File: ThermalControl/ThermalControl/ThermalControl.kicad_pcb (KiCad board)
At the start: 2 copper layers, 75 x 49 mm, 24 parts, among them J1 12V, J2 GND, J3 DC IN, J4 5V, U1 NODE_MCU, U2 RELAY MOD

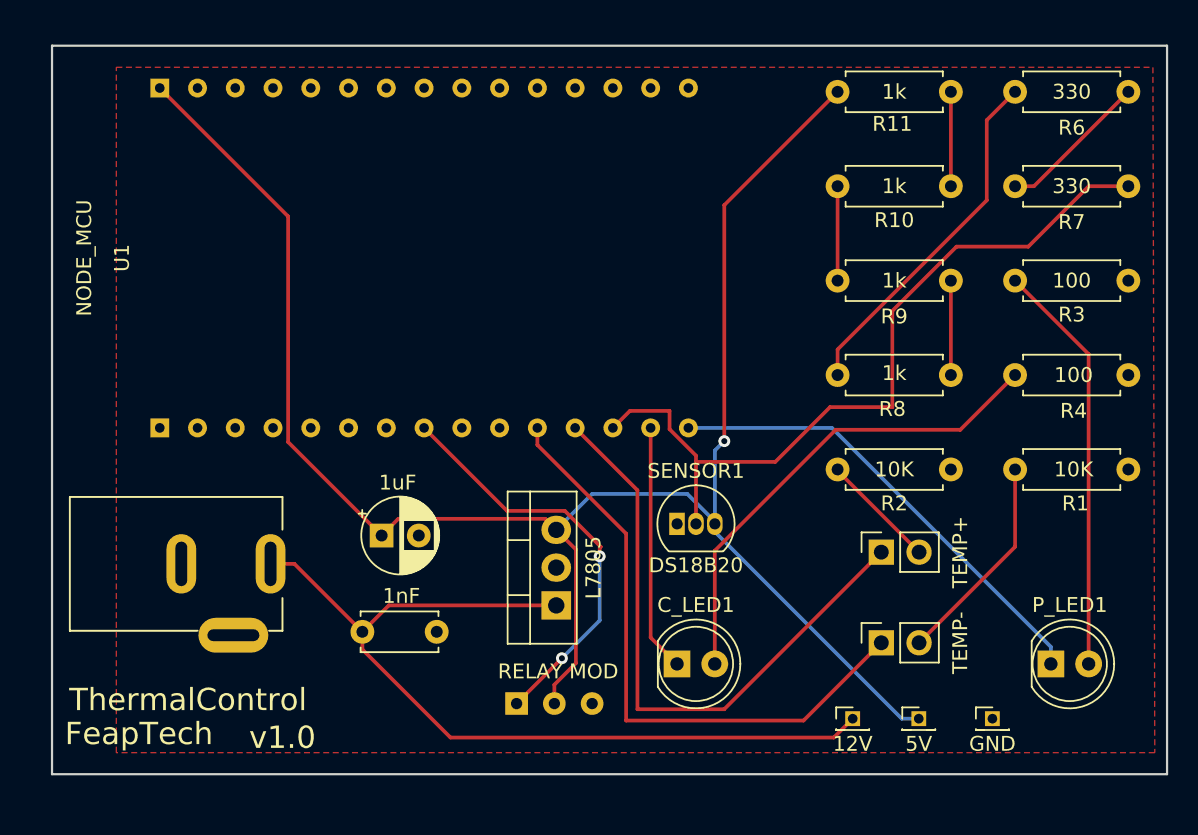
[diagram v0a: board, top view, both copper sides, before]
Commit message: project ready to production
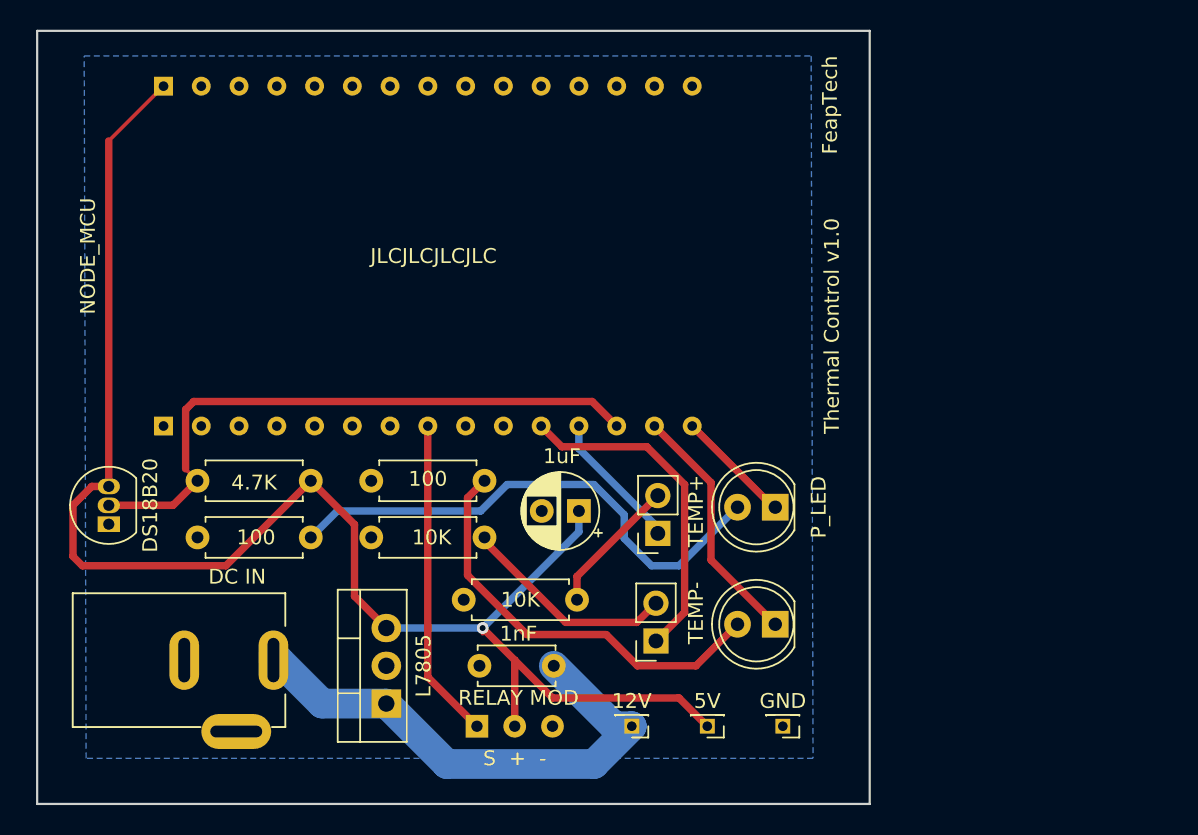
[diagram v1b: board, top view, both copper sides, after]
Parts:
- removed R10, R11, R8, R9: 1k, Resistor_THT:R_Axial_DIN0207_L6.3mm_D2.5mm_P7.62mm_Horizontal
- removed R6, R7: 330, Resistor_THT:R_Axial_DIN0207_L6.3mm_D2.5mm_P7.62mm_Horizontal
- added R5: 100, Resistor_THT:R_Axial_DIN0207_L6.3mm_D2.5mm_P7.62mm_Horizontal, F.Cu at (73.4, 76.1)
- C1: value 1uF -> 1nF; footprint Capacitor_THT:CP_Radial_D5.0mm_P2.50mm -> Capacitor_THT:C_Disc_D5.0mm_W2.5mm_P5.00mm
- C2: value 1nF -> 1uF; footprint Capacitor_THT:C_Disc_D5.0mm_W2.5mm_P5.00mm -> Capacitor_THT:CP_Radial_D5.0mm_P2.50mm
- C_LED1: value LED -> C_LED
- J1: value 12V -> 5V
- J4: value 5V -> 12V
- R3: value 100 -> 4.7K
- moved R3 56.6 mm to (65.8, 72.3)
- moved SENSOR1 38.2 mm to (59.8, 75.2), turned to 90 degrees
- moved R4 36.4 mm to (85.1, 72.3), turned to 180 degrees
- moved R1 30.7 mm to (91.3, 80.3), turned to 180 degrees
- moved R2 24.2 mm to (85.1, 76.1), turned to 180 degrees
- moved P_LED1 21.3 mm to (104.6, 74.0), turned to 180 degrees
- moved J4 19.3 mm to (95.0, 88.8), turned to 180 degrees
- moved C2 16.7 mm to (91.4, 74.3), turned to 180 degrees
- moved BTN2 15.2 mm to (96.6, 83.0), turned to 180 degrees
- moved BTN1 15.1 mm to (96.7, 75.8), turned to 180 degrees
- moved C1 14.5 mm to (89.7, 84.7), turned to 180 degrees
- moved J2 14.1 mm to (105.2, 88.8), turned to 180 degrees
- moved Vreg1 13.2 mm to (78.5, 87.2)
- moved J1 9.79 mm to (100.1, 88.8), turned to 180 degrees
- moved C_LED1 7.13 mm to (104.6, 81.9), turned to 180 degrees
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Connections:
- J3 pad 4: Net-(C2-Pad1) -> Net-(C1-Pad1)
- R1 pad 1: Net-(BTN2-Pad2) -> Net-(BTN1-Pad2)
- R2 pad 1: Net-(BTN1-Pad2) -> Net-(BTN2-Pad2)
- R3 pad 1: Net-(P_LED1-Pad2) -> Net-(R3-Pad1)
- R3 pad 2: GND -> Net-(C2-Pad1)
- SENSOR1 pad 2: Net-(R7-Pad2) -> Net-(R3-Pad1)
- SENSOR1 pad 3: Net-(C1-Pad1) -> Net-(C2-Pad1)
- U1 pad 1: Net-(C1-Pad1) -> Net-(C2-Pad1)
- U1 pad 28: Net-(R7-Pad2) -> Net-(R3-Pad1)
- U2 pad 2: Net-(C1-Pad1) -> Net-(C2-Pad1)
- Vreg1 pad 1: Net-(C2-Pad1) -> Net-(C1-Pad1)
- Vreg1 pad 3: Net-(C1-Pad1) -> Net-(C2-Pad1)
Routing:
- net Net-(C1-Pad1): track 126.6 -> 35.1 mm, vias 1 -> 0
- net Net-(R7-Pad2): track 53.2 -> 0.00 mm
- net Net-(C2-Pad1): track 59.0 -> 105.2 mm, vias 0 -> 1
- net Net-(R3-Pad1): track 0.00 -> 41.7 mm
- net Net-(BTN1-Pad1): track 41.4 -> 9.42 mm
- net Net-(R6-Pad1): track 24.0 -> 0.00 mm
- net Net-(P_LED1-Pad1): track 31.6 -> 7.85 mm
- net Net-(BTN2-Pad1): track 41.5 -> 22.6 mm
- net Net-(R6-Pad2): track 10.3 -> 0.00 mm
- net Net-(P_LED1-Pad2): track 27.8 -> 35.0 mm
- net Net-(U1-Pad23): track 28.1 -> 21.6 mm, vias 2 -> 0
- net Net-(R10-Pad2): track 6.35 -> 0.00 mm
- net Net-(R10-Pad1): track 6.35 -> 0.00 mm
- net Net-(R8-Pad2): track 6.35 -> 0.00 mm
- net Net-(C_LED1-Pad2): track 32.7 -> 28.7 mm
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- added copper zone on B.Cu, net GND
- removed copper zone on F.Cu, net GND
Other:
- board size 75 x 49 mm -> 56 x 52 mm
- board text added: "JLCJLCJLCJLC"
- board text added: "P_LED"
- board text added: "Thermal Control v1.0"
- board text removed: "ThermalControl"
- board text removed: "v1.0"
